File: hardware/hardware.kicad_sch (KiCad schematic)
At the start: 18 parts, among them J1 Screw_Terminal_01x02, J2 Screw_Terminal_01x02, J3 Screw_Terminal_01x02, K1 RM85-2011-35-1005, K2 RM85-2011-35-1005, Q1 BC337, Q2 BC337, U1 XIAO-ESP32-C6, U2 DS18B20

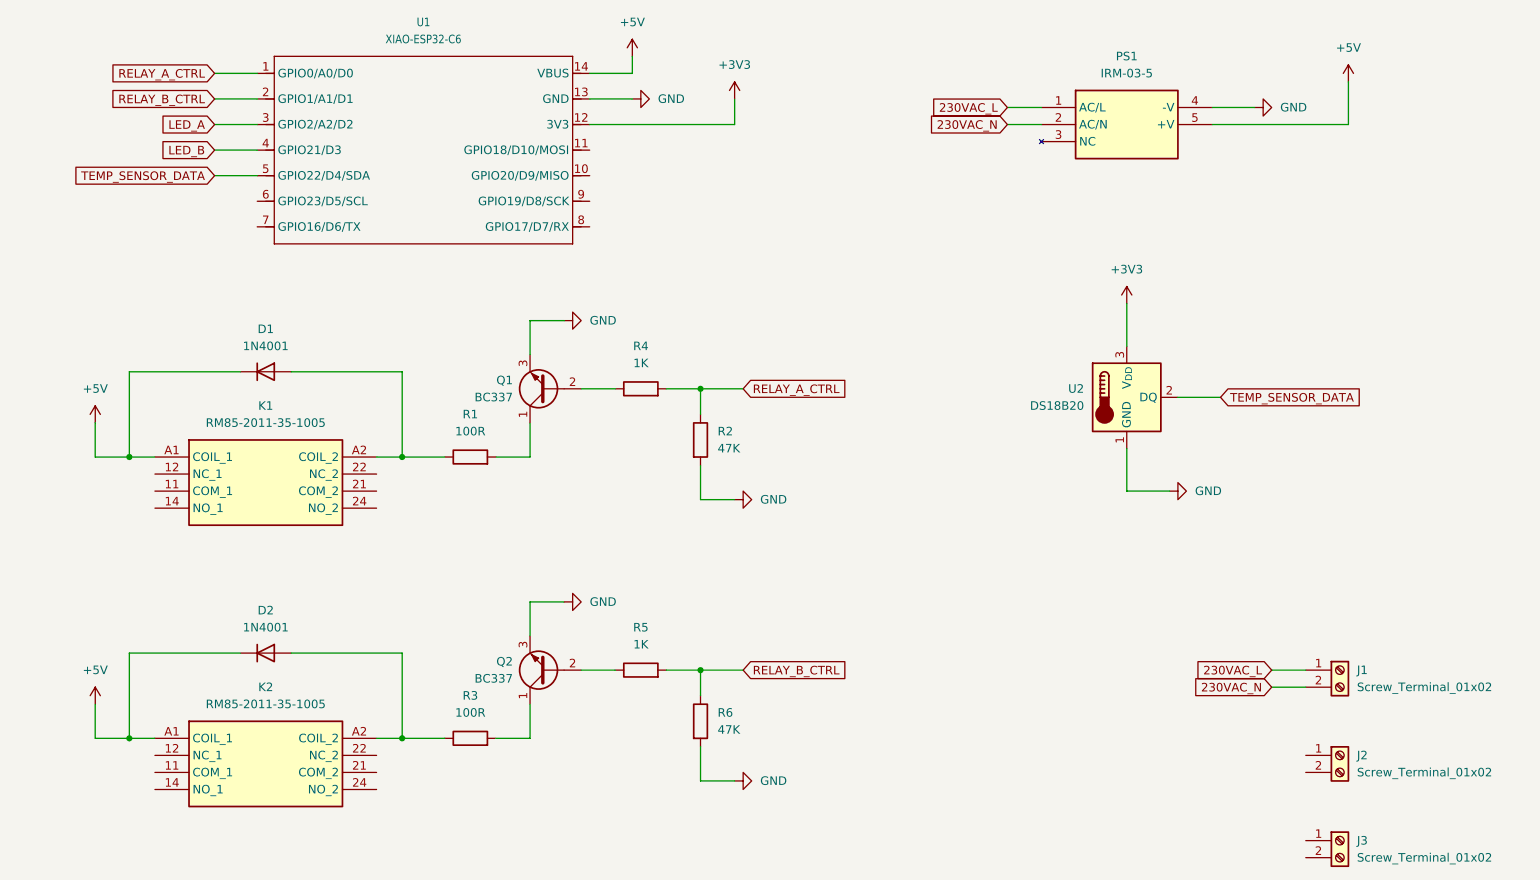
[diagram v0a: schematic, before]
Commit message: Started working on new PCB layout
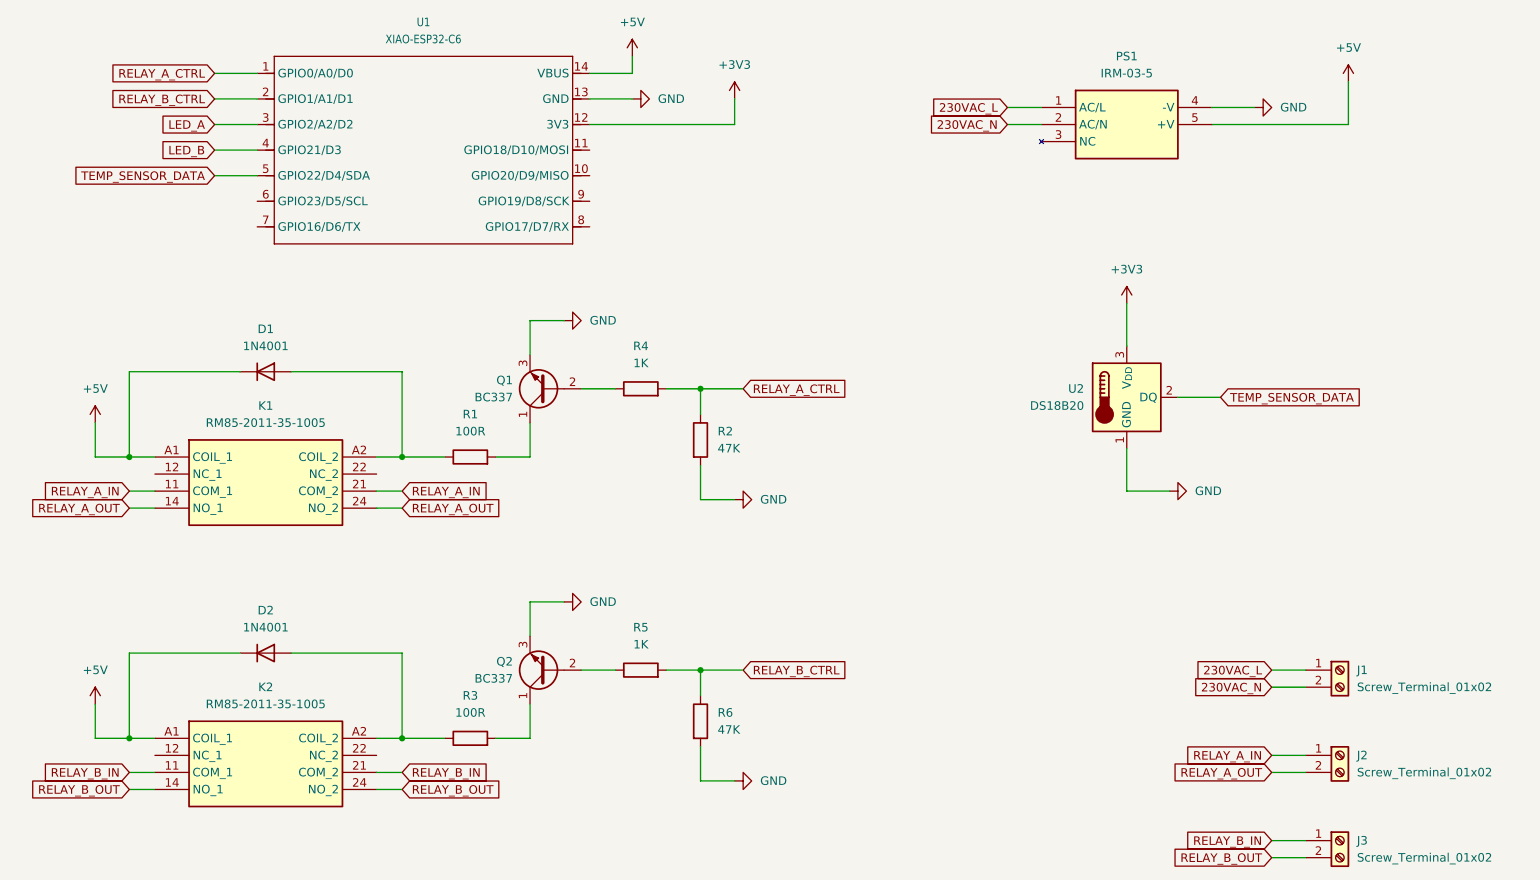
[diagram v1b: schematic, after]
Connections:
- net RELAY_B_IN: now reaches K2.11 (COM_1)
- net RELAY_B_IN: now also J3.1 (Pin_1), K2.21 (COM_2)
- net RELAY_B_OUT: now reaches K2.14 (NO_1)
- net RELAY_B_OUT: now also J3.2 (Pin_2), K2.24 (NO_2)
- net RELAY_A_IN: now reaches J2.1 (Pin_1)
- net RELAY_A_IN: now also K1.11 (COM_1), K1.21 (COM_2)
- net RELAY_A_OUT: now reaches J2.2 (Pin_2)
- net RELAY_A_OUT: now also K1.14 (NO_1), K1.24 (NO_2)
